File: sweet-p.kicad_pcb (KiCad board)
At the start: 2 copper layers, 68.1 x 69 mm, 12 parts, among them J1 Screw_Terminal_01x03, J2 Screw_Terminal_01x02, J3 Conn_01x04_Female, J4 Screw_Terminal_01x04, J5 Conn_01x06_Female, J6 Conn_01x08_Female, U1 RFM95W-868S2, U2 Adafruit-Mini-GPS

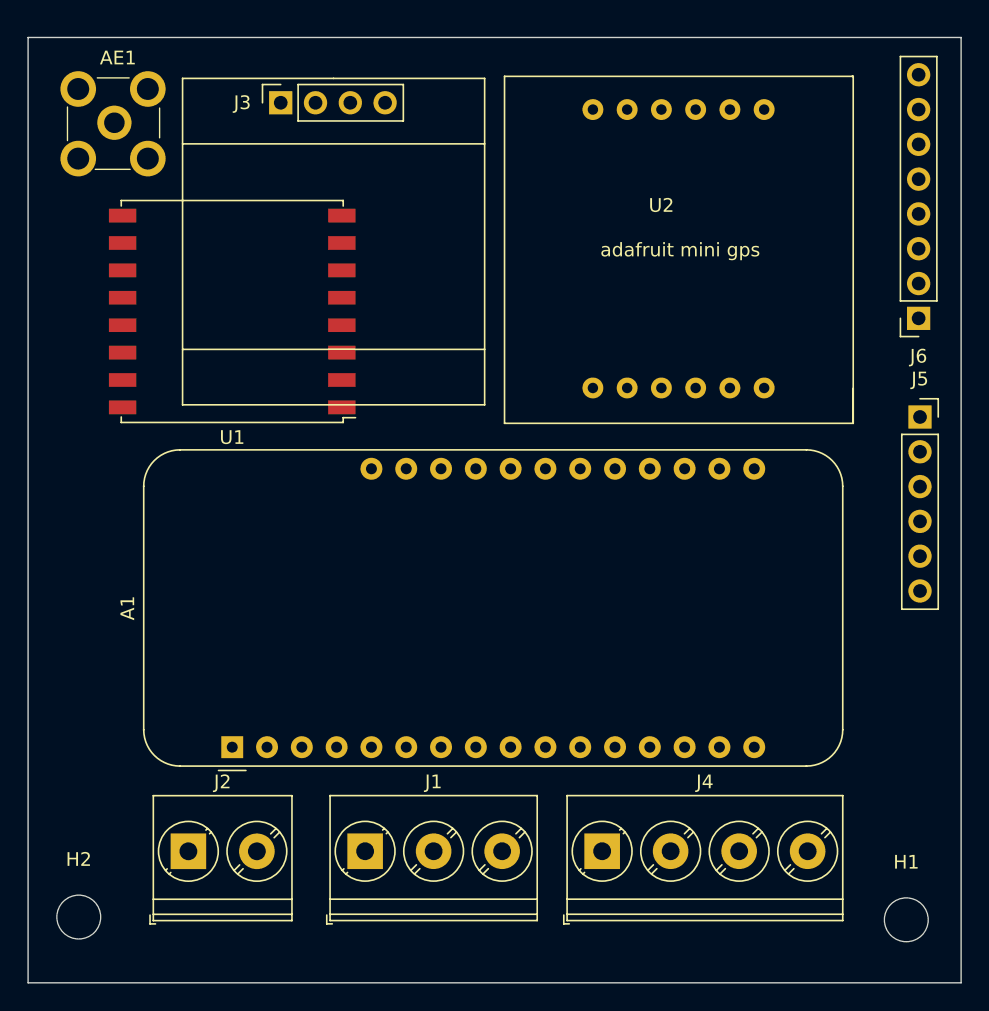
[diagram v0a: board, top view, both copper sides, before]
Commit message: update
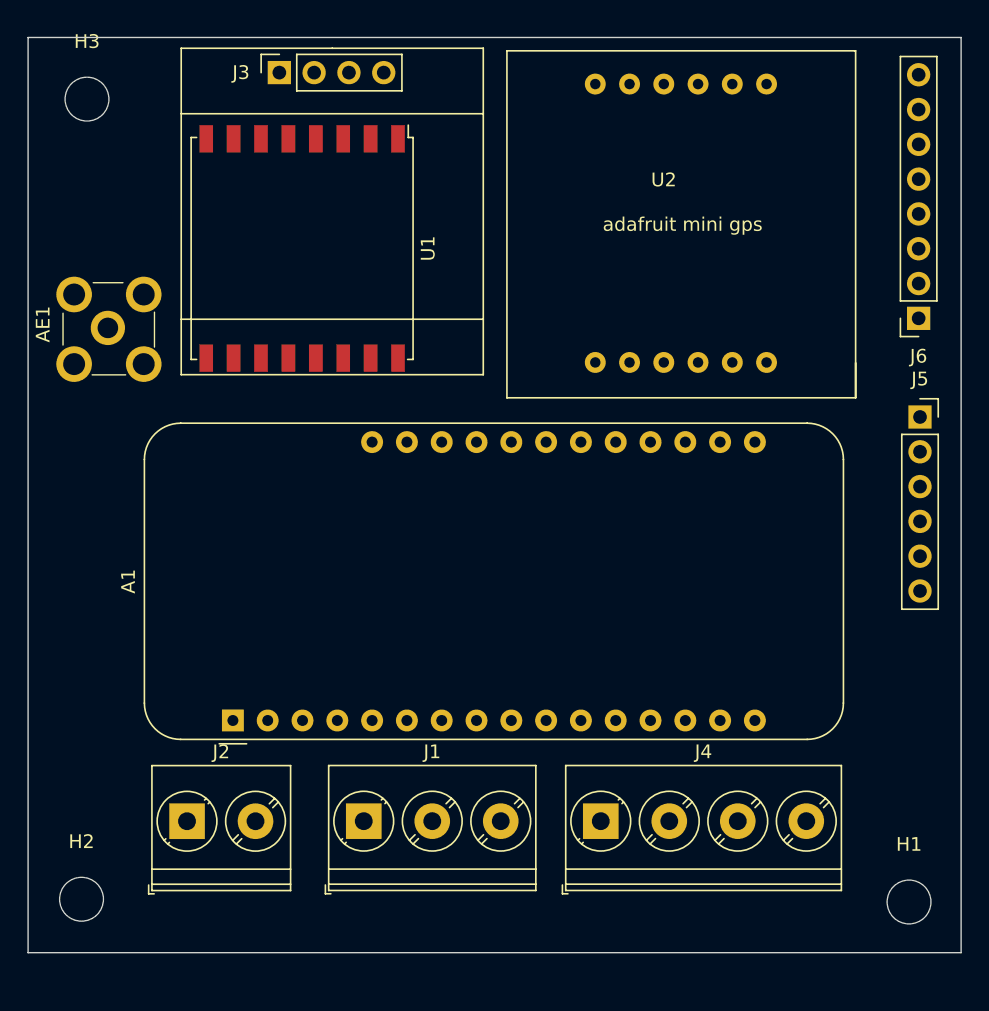
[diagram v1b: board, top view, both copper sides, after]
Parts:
- added H3: MountingHole, MountingHole:MountingHole_3.2mm_M3, F.Cu at (167.0, 61.1)
- moved AE1 15.0 mm to (168.6, 77.9), turned to 90 degrees
- moved U1 6.87 mm to (182.7, 72.0), turned to -90 degrees
- moved J3 2.20 mm to (181.0, 59.2)
- moved J1 2.20 mm to (187.2, 113.8)
- moved J4 2.20 mm to (204.5, 113.8)
- moved J2 2.20 mm to (174.3, 113.8)
- moved A1 1.95 mm to (177.7, 106.5)
- moved U2 1.87 mm to (216.6, 60.0)
- moved H1 1.32 mm to (227.0, 119.7)
- moved H2 1.32 mm to (166.6, 119.5)
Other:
- board size 68.1 x 69 mm -> 68.1 x 66.8 mm
